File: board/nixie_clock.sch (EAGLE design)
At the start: 40 parts, among them U1 AMS1117-5.0, U2 SN74141N

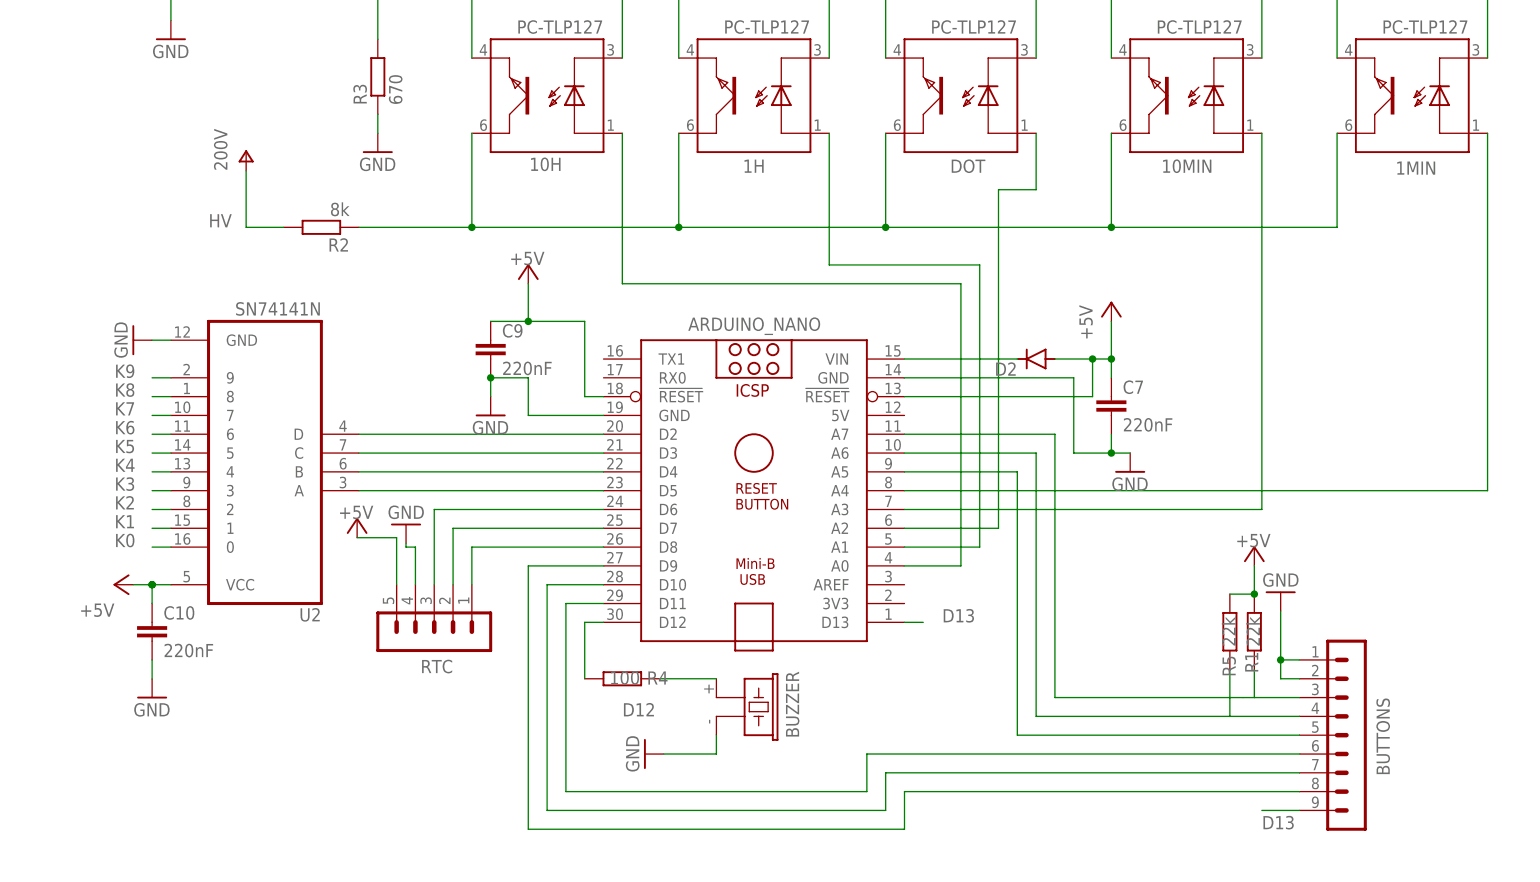
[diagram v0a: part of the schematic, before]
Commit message: board design v3
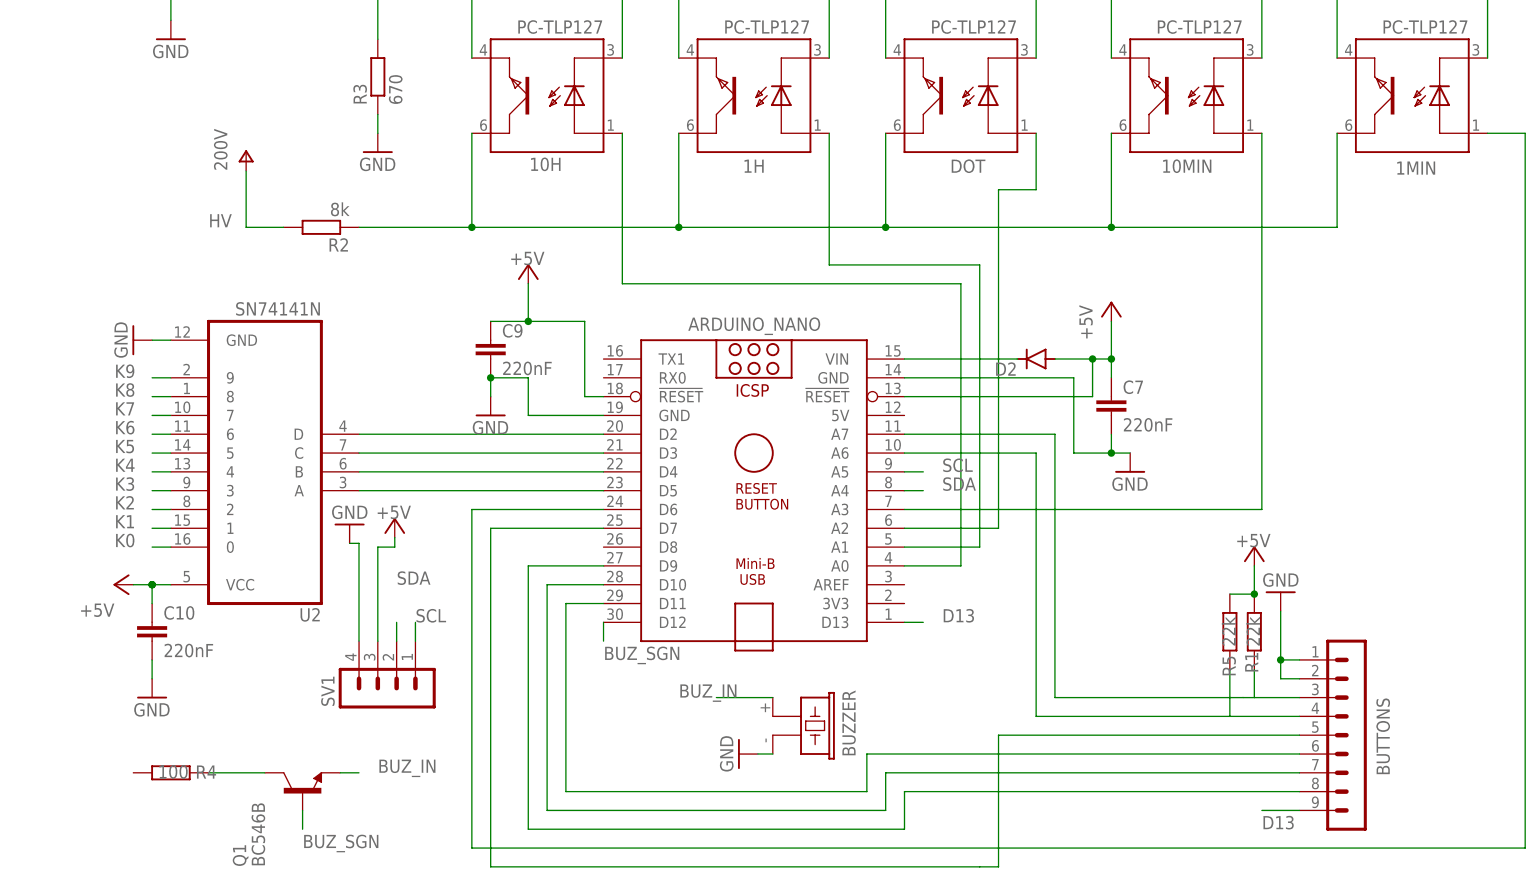
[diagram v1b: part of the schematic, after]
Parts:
- removed RTC: (no value), con-lstb:MA05-1
- added Q1: BC546B, transistor-npn:BC546B
- added SV1: (no value), con-lstb:MA04-1
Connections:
- removed net D12: BUZZER.1, R4.2
- removed net N$17: ARDUINO_NANO.A5, BUTTONS.5
- removed net N$29: 1MIN.A, ARDUINO_NANO.A4
- removed net N$8: ARDUINO_NANO.D12, R4.1
- new net BUZ_IN: BUZZER.1, Q1.E
- new net BUZ_SGN: ARDUINO_NANO.D12, Q1.B
- new net SCL: ARDUINO_NANO.A5, SV1.1
- new net SDA: ARDUINO_NANO.A4, SV1.2
- net +5V: now also SV1.3; no longer RTC.5
- net GND: now also SV1.4; no longer RTC.4
- net N$3: now also 1MIN.A, ARDUINO_NANO.D6; no longer ARDUINO_NANO.D8, RTC.1
- net N$4: now also BUTTONS.5; no longer RTC.2
- net N$7: now also Q1.C, R4.2; no longer ARDUINO_NANO.D6, RTC.3
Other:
- moved on the sheet: BUZZER, R4
